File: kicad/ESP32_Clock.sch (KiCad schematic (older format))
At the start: 1 part

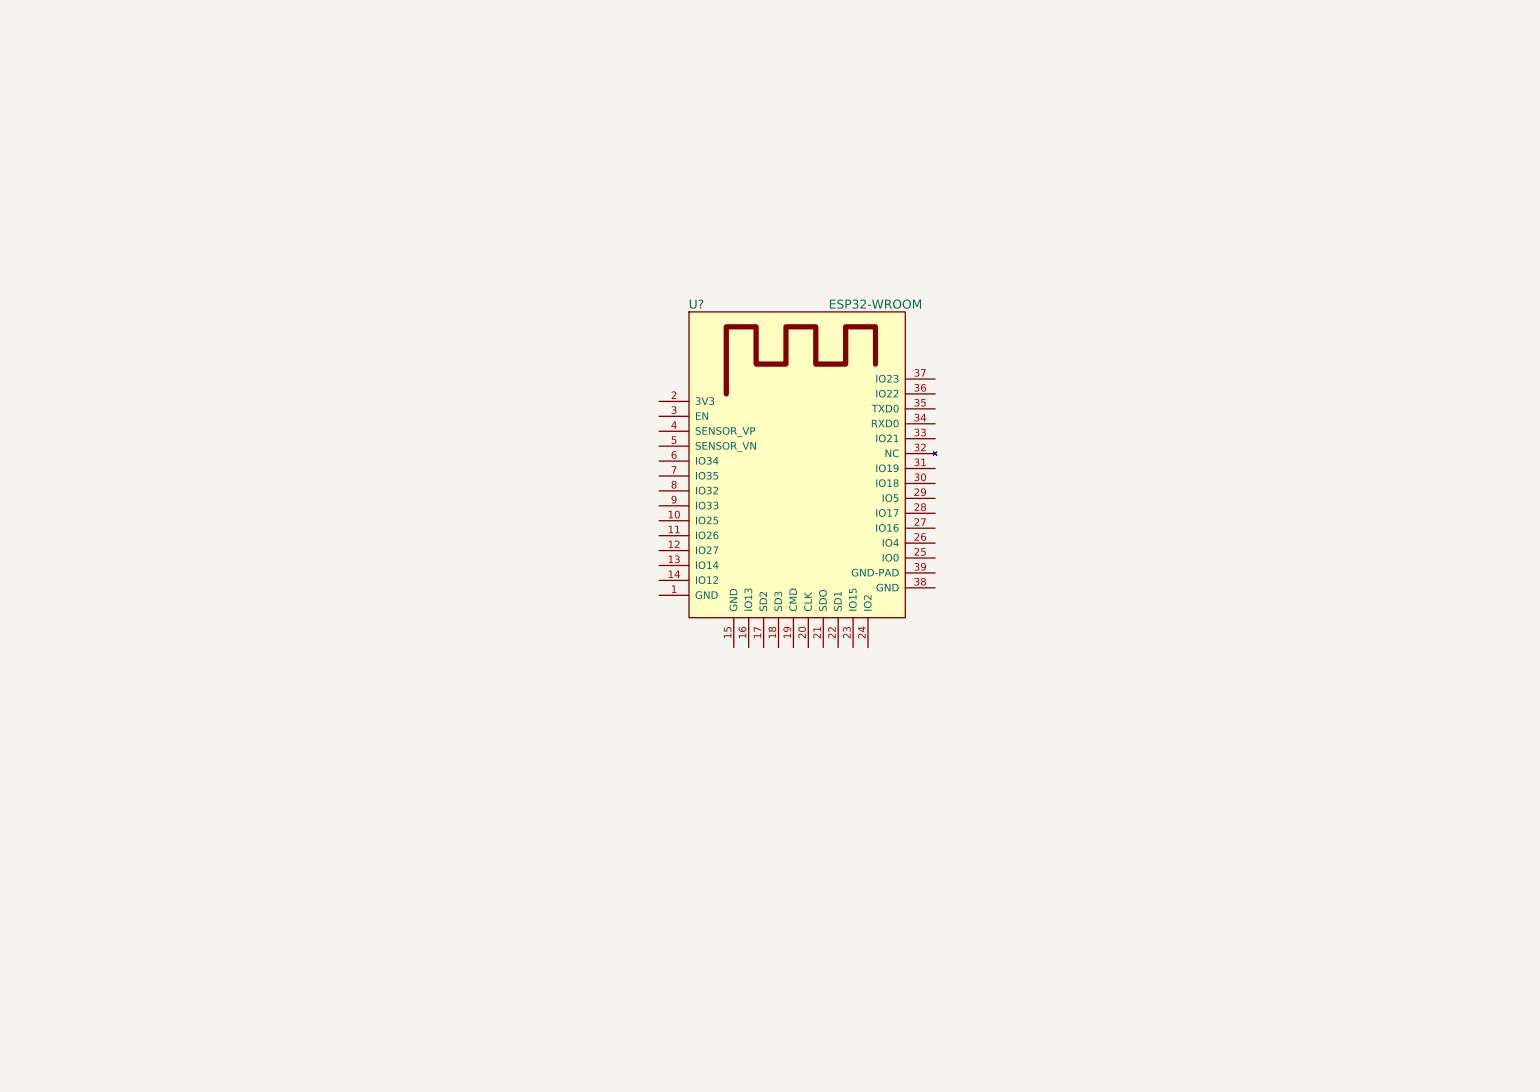
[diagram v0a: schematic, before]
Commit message: Board design almost ready for fabrication
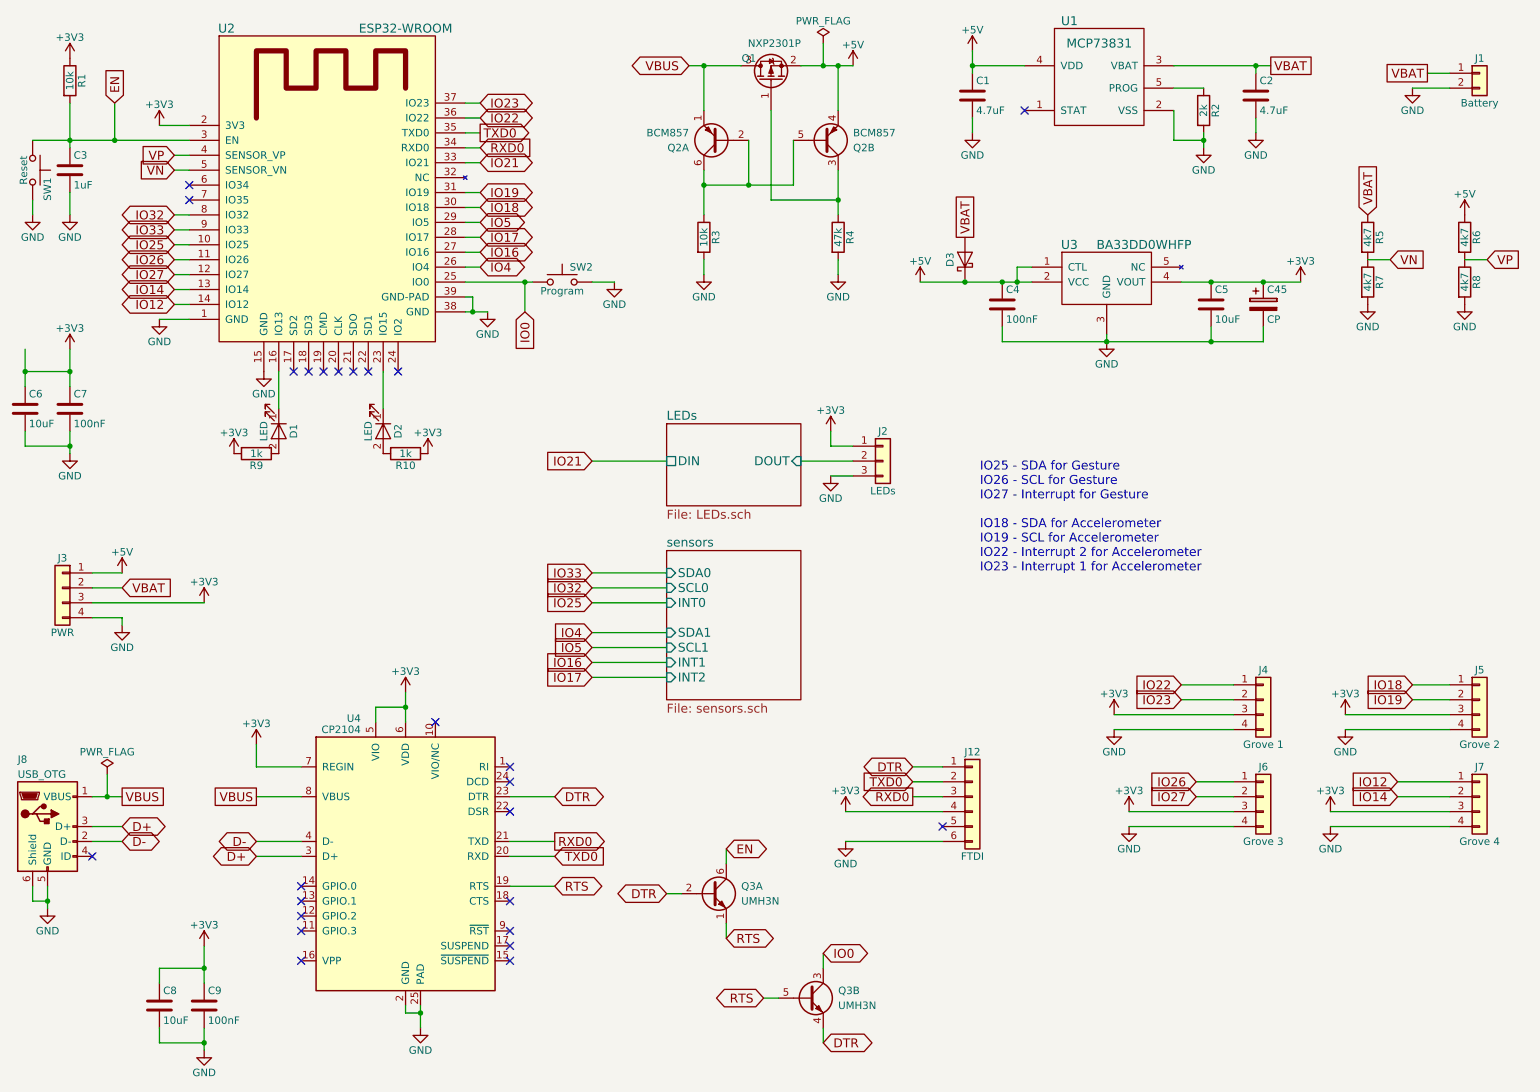
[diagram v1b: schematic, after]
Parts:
- added C1, C2: 4.7uF, Capacitors_SMD:C_0805_HandSoldering, symbol C
- added C3: 1uF, Capacitors_SMD:C_0805_HandSoldering, symbol C
- added C4, C7, C9: 100nF, Capacitors_SMD:C_0603_HandSoldering, symbol C
- added C45: CP, Capacitors_THT:CP_Radial_D8.0mm_P3.50mm, symbol CP
- added C5, C6, C8: 10uF, Capacitors_SMD:C_0805_HandSoldering, symbol C
- added D1, D2: LED, LEDs:LED_0603_HandSoldering, symbol LED
- added D3: (no value), Diodes_SMD:D_SMA_Handsoldering, symbol D_Schottky
- added J1: Battery, Connectors_JST:JST_PH_S2B-PH-K_02x2.00mm_Angled, symbol Conn_01x02
- added J12: FTDI, Pin_Headers:Pin_Header_Straight_1x06_Pitch2.54mm, symbol Conn_01x06
- added J2: LEDs, Pin_Headers:Pin_Header_Straight_1x03_Pitch2.54mm, symbol Conn_01x03
- added J3: PWR, Pin_Headers:Pin_Header_Straight_1x04_Pitch2.54mm, symbol Conn_01x04
- added J4: Grove 1, Pin_Headers:Pin_Header_Straight_1x04_Pitch2.54mm, symbol Conn_01x04
- added J5: Grove 2, Pin_Headers:Pin_Header_Straight_1x04_Pitch2.54mm, symbol Conn_01x04
- added J6: Grove 3, Pin_Headers:Pin_Header_Straight_1x04_Pitch2.54mm, symbol Conn_01x04
- added J7: Grove 4, Pin_Headers:Pin_Header_Straight_1x04_Pitch2.54mm, symbol Conn_01x04
- added J8: USB_OTG, MicroUSB_Custom:MicroUSB, symbol USB_OTG
- added Q1: NXP2301P, TO_SOT_Packages_SMD:SOT-23, symbol BSS83P
- added Q2: BCM857, TO_SOT_Packages_SMD:SOT-363_SC-70-6_Handsoldering, symbol Q_DUAL_PNP_PNP_E1B1C2E2B2C1
- added Q3: UMH3N, TO_SOT_Packages_SMD:SOT-363_SC-70-6_Handsoldering, symbol Q_DUAL_NPN_NPN_E1B1C2E2B2C1
- added R1, R3: 10k, Resistors_SMD:R_0603_HandSoldering, symbol R
- added R10, R9: 1k, Resistors_SMD:R_0603_HandSoldering, symbol R
- added R2: 2k, Resistors_SMD:R_0603_HandSoldering, symbol R
- added R4: 47k, Resistors_SMD:R_0603_HandSoldering, symbol R
- added R5, R6, R7, R8: 4k7, Resistors_SMD:R_0603_HandSoldering, symbol R
- added SW1: Reset, Buttons_Switches_SMD:SW_SPST_EVPBF, symbol SW_Push
- added SW2: Program, Buttons_Switches_SMD:SW_SPST_EVPBF, symbol SW_Push
- added U1: MCP73831, TO_SOT_Packages_SMD:SOT-23-5_HandSoldering, symbol MCP73831
- added U3: BA33DD0WHFP, LDO:LDO, symbol BA33DD0WHFP
- added U4: CP2104, QFN-24:QFN-24, symbol CP2104
- gave numbers to parts that had none: 1
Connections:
- net GND: now reaches U2.1 (GND)
- net GND: now also U2.15 (GND), U2.38 (GND), U2.39 (GND-PAD), C1.2, C2.2, C3.2, C4.2, C45.2, C5.2, C6.2, C7.2, C8.2, C9.2, J1.2 (Pin_2), J12.6 (Pin_6), J2.3 (Pin_3), J3.4 (Pin_4), J4.4 (Pin_4), J5.4 (Pin_4), J6.4 (Pin_4), J7.4 (Pin_4), J8.5 (GND), J8.6 (Shield), R2.2, R3.2, R4.2, R7.2, R8.2, SW1.2, SW2.2, U1.2 (VSS), U3.3 (GND), U4.2 (GND), U4.25 (PAD)
- net IO25: now reaches U2.10 (IO25)
- net IO26: now reaches U2.11 (IO26)
- net IO26: now also J6.1 (Pin_1)
- net IO27: now reaches U2.12 (IO27)
- net IO27: now also J6.2 (Pin_2)
- net IO14: now reaches U2.13 (IO14)
- net IO14: now also J7.2 (Pin_2)
- net IO12: now reaches U2.14 (IO12)
- net IO12: now also J7.1 (Pin_1)
- net at U2.16 (IO13): now also D1.1 (K)
- net +3V3: now reaches U2.2 (3V3)
- net +3V3: now also C45.1, C5.1, C6.1, C7.1, C8.1, C9.1, J12.4 (Pin_4), J2.1 (Pin_1), J3.3 (Pin_3), J4.3 (Pin_3), J5.3 (Pin_3), J6.3 (Pin_3), J7.3 (Pin_3), R1.1, R10.1, R9.2, U3.4 (VOUT), U4.5 (VIO), U4.6 (VDD), U4.7 (REGIN)
- net at U2.23 (IO15): now also D2.1 (K)
- net IO0: now reaches U2.25 (IO0)
- net IO0: now also Q3.3 (C2), SW2.1
- net IO4: now reaches U2.26 (IO4)
- net IO16: now reaches U2.27 (IO16)
- net IO17: now reaches U2.28 (IO17)
- net IO5: now reaches U2.29 (IO5)
- net EN: now reaches U2.3 (EN)
- net EN: now also C3.1, Q3.6 (C1), R1.2, SW1.1
- net IO18: now reaches U2.30 (IO18)
- net IO18: now also J5.1 (Pin_1)
- net IO19: now reaches U2.31 (IO19)
- net IO19: now also J5.2 (Pin_2)
- net IO21: now reaches U2.33 (IO21)
- net RXD0: now reaches U2.34 (RXD0)
- net RXD0: now also J12.3 (Pin_3), U4.21 (TXD)
- net TXD0: now reaches U2.35 (TXD0)
- net TXD0: now also J12.2 (Pin_2), U4.20 (RXD)
- net IO22: now reaches U2.36 (IO22)
- net IO22: now also J4.1 (Pin_1)
- net IO23: now reaches U2.37 (IO23)
- net IO23: now also J4.2 (Pin_2)
- net VP: now reaches U2.4 (SENSOR_VP)
- net VP: now also R6.2, R8.1
- net VN: now reaches U2.5 (SENSOR_VN)
- net VN: now also R5.2, R7.1
- net IO32: now reaches U2.8 (IO32)
- net IO33: now reaches U2.9 (IO33)
- new net: Q2.2 (B1), Q2.5 (B2), Q2.6 (C1), R3.1
- new net: Q1.1 (G), Q2.3 (C2), R4.1
- new net: R2.1, U1.5 (PROG)
- new net: D1.2 (A), R9.1
- new net: D2.2 (A), R10.2
- new net +5V: C1.1, C4.1, D3.1 (K), J3.1 (Pin_1), Q1.2 (S), Q2.4 (E2), R6.1, U1.4 (VDD), U3.1 (CTL), U3.2 (VCC)
- new net D+: J8.3 (D+), U4.3 (D+)
- new net D-: J8.2 (D-), U4.4 (D-)
- new net DTR: J12.1 (Pin_1), Q3.2 (B1), Q3.4 (E2), U4.23 (DTR)
- new net LEDs/DOUT: J2.2 (Pin_2)
- new net RTS: Q3.1 (E1), Q3.5 (B2), U4.19 (RTS)
- new net VBAT: C2.1, D3.2 (A), J1.1 (Pin_1), J3.2 (Pin_2), R5.1, U1.3 (VBAT)
- new net VBUS: J8.1 (VBUS), Q1.3 (D), Q2.1 (E1), U4.8 (VBUS)
- no-connect marks 0 -> 25
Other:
- note added: "IO25 - SDA for Gesture\nIO26 - SCL for Gesture\nIO27 - Interrupt for Gesture\n\nIO18 - SDA for Accelerometer\nIO19 - SCL for Accelerometer\nIO22 - Interrupt 2 for Accelerometer\nIO23 - Interrupt 1 for Accelerometer"
- moved on the sheet: U2
